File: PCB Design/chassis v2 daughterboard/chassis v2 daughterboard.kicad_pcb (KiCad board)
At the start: 2 copper layers, 191.3 x 26.5 mm, 89 parts, among them CN1 microblade connector, CN10 std 2 pin 2.54mm pitch, CN11 microblade connector, CN12 std 2 pin 2.54mm pitch, CN13 microblade connector, CN14 std 2 pin 2.54mm pitch, CN15 microblade connector, CN16 std 2 pin 2.54mm pitch, CN17 microblade connector, CN18 std 2 pin 2.54mm pitch, CN19 microblade connector, CN2 std 2 pin 2.54mm pitch, CN20 std 2 pin 2.54mm pitch, CN21 microblade connector, CN22 std 2 pin 2.54mm pitch, CN23 microblade connector, CN24 std 2 pin 2.54mm pitch, CN25 microblade connector, CN26 std 2 pin 2.54mm pitch, CN27 microblade connector, CN28 std 2 pin 2.54mm pitch, CN29 microblade connector, CN3 microblade connector, CN30 std 2 pin 2.54mm pitch, CN31 microblade connector, CN32 std 2 pin 2.54mm pitch, CN4 std 2 pin 2.54mm pitch, CN5 microblade connector, CN6 std 2 pin 2.54mm pitch, CN7 microblade connector, CN8 std 2 pin 2.54mm pitch, CN9 microblade connector, J1 socket, J2 Conn_02x04_Odd_Even, J3 Conn_02x04_Odd_Even, J4 pins, Q1 NMOS, Q10 NMOS, Q11 NMOS, Q12 NMOS, Q13 NMOS, Q14 NMOS, Q15 NMOS, Q16 NMOS, Q2 NMOS, Q3 NMOS, Q4 NMOS, Q5 NMOS, Q6 NMOS, Q7 NMOS, Q8 NMOS, Q9 NMOS, U1 74HC595, U2 74HC595

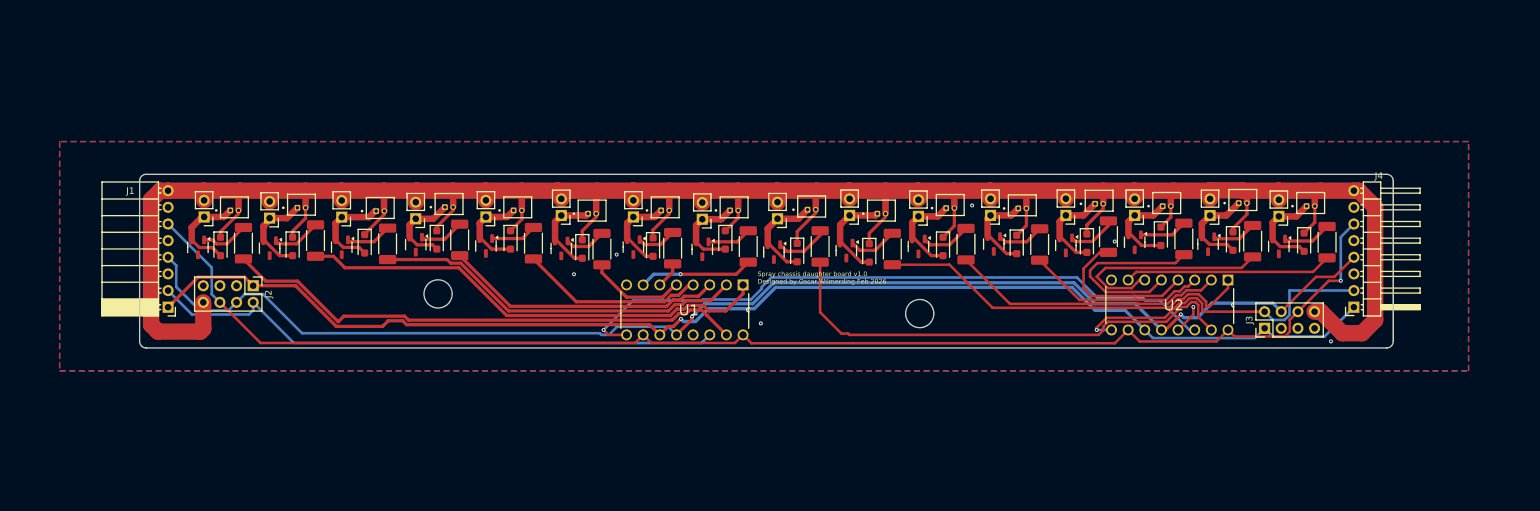
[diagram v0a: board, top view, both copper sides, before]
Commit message: stable somewhat
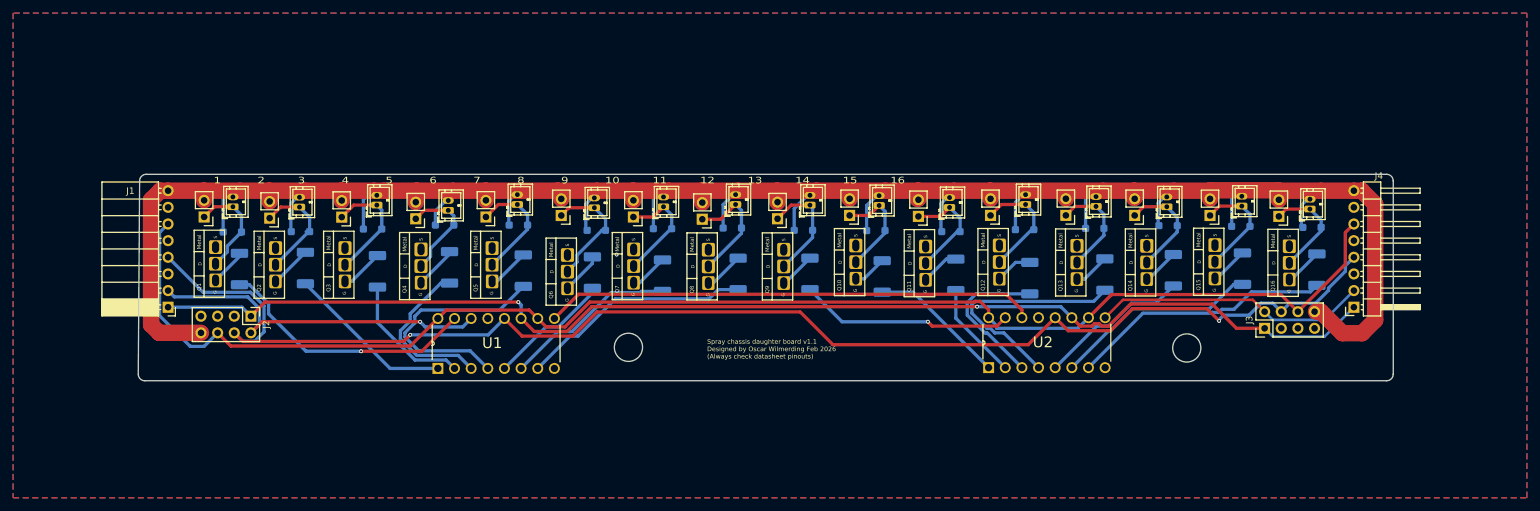
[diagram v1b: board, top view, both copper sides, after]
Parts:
- removed ?: , 
- removed G***: LOGO, custom footprints:graphic
- added REF**: MountingHole_4.3mm_M4, MountingHole:MountingHole_4.3mm_M4, F.Cu at (212.0, 106.5)
- CN1, CN11, CN13, CN15, CN17, CN19, CN21, CN23, CN25, CN27, CN29, CN3, CN31, CN5, CN7, CN9: footprint custom footprints:MOLEX_53047-0210_test -> chassis v2 primary board:modified jst zh used
- D1, D10, D11, D12, D13, D14, D15, D16, D2, D3, D4, D5, D6, D7, D8, D9, R1, R10, R11, R12, R13, R14, R15, R16, R2, R3, R4, R5, R6, R7, R8, R9: moved to B.Cu
- Q1, Q10, Q11, Q12, Q13, Q14, Q15, Q16, Q2, Q3, Q4, Q5, Q6, Q7, Q8, Q9: footprint Package_TO_SOT_SMD:SOT-23-3 -> chassis v2 primary board:Big Mosfet Old Style
- moved REF** 30.2 mm to (126.8, 106.4)
- moved U1 11.3 mm to (115.5, 102.0), turned to 90 degrees
- moved Q6 6.15 mm to (117.5, 97.4), turned to 90 degrees
- moved Q14 5.91 mm to (205.9, 96.0), turned to 90 degrees
- moved Q4 5.86 mm to (95.1, 96.5), turned to 90 degrees
- moved R13 5.81 mm to (199.5, 95.3)
- moved Q1 5.72 mm to (63.8, 96.2), turned to 90 degrees
- moved Q5 5.48 mm to (106.0, 96.3), turned to 90 degrees
- moved Q7 5.44 mm to (127.6, 96.5), turned to 90 degrees
- moved Q13 5.41 mm to (195.2, 96.0), turned to 90 degrees
- moved Q12 5.36 mm to (183.4, 95.9), turned to 90 degrees
- moved R12 5.35 mm to (188.1, 95.8)
- moved Q15 5.32 mm to (216.3, 95.9), turned to 90 degrees
- moved Q16 5.29 mm to (227.7, 96.0), turned to 90 degrees
- moved Q3 5.24 mm to (83.5, 96.3), turned to 90 degrees
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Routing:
- net /mosfet subsystem2/sig in: track 72.4 -> 25.6 mm
- net /mosfet subsystem9/sig in: track 74.0 -> 32.6 mm, vias 0 -> 1
- net /mosfet subsystem1/sig in: track 80.5 -> 40.0 mm, vias 0 -> 1
- net /mosfet subsystem10/sig in: track 58.4 -> 21.0 mm
- net /mosfet subsystem3/sig in: track 56.6 -> 20.1 mm
- net Net-(J1-Pin_2): track 88.7 -> 54.5 mm, vias 0 -> 1
- net +12V: track 396.9 -> 369.2 mm
- net /mosfet subsystem11/sig in: track 41.7 -> 14.9 mm
- net Net-(U1-QH'): track 101.1 -> 75.0 mm, vias 1 -> 0
- net /mosfet subsystem7/sig in: track 4.02 -> 26.5 mm
- net /mosfet subsystem8/sig in: track 17.5 -> 35.6 mm, vias 1 -> 0
- net /mosfet subsystem4/sig in: track 42.7 -> 25.1 mm
- net /mosfet subsystem13/sig in: track 23.7 -> 36.2 mm
- net Net-(J1-Pin_4): track 203.5 -> 215.5 mm
- net +3V3: track 207.7 -> 219.6 mm, vias 1 -> 0
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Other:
- board size 191.3 x 26.5 mm -> 191.5 x 31.5 mm
- board text added: "1 2 3 4 5 6 7 8 9 10 11 12 13 14 15 16"
- board text added: "Spray chassis daughter board v1.1 Designed by Oscar Wilmerding Feb 2026 (Always check datasheet pinouts)"
- board text removed: "Spray chassis daughter board v1.0 Designed by Oscar Wilmerding Feb 2026"
